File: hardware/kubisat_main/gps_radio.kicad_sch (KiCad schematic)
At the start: 10 parts, among them J1 IPX, U2 NEO-6M-GPS, U5 XL1278-SMT

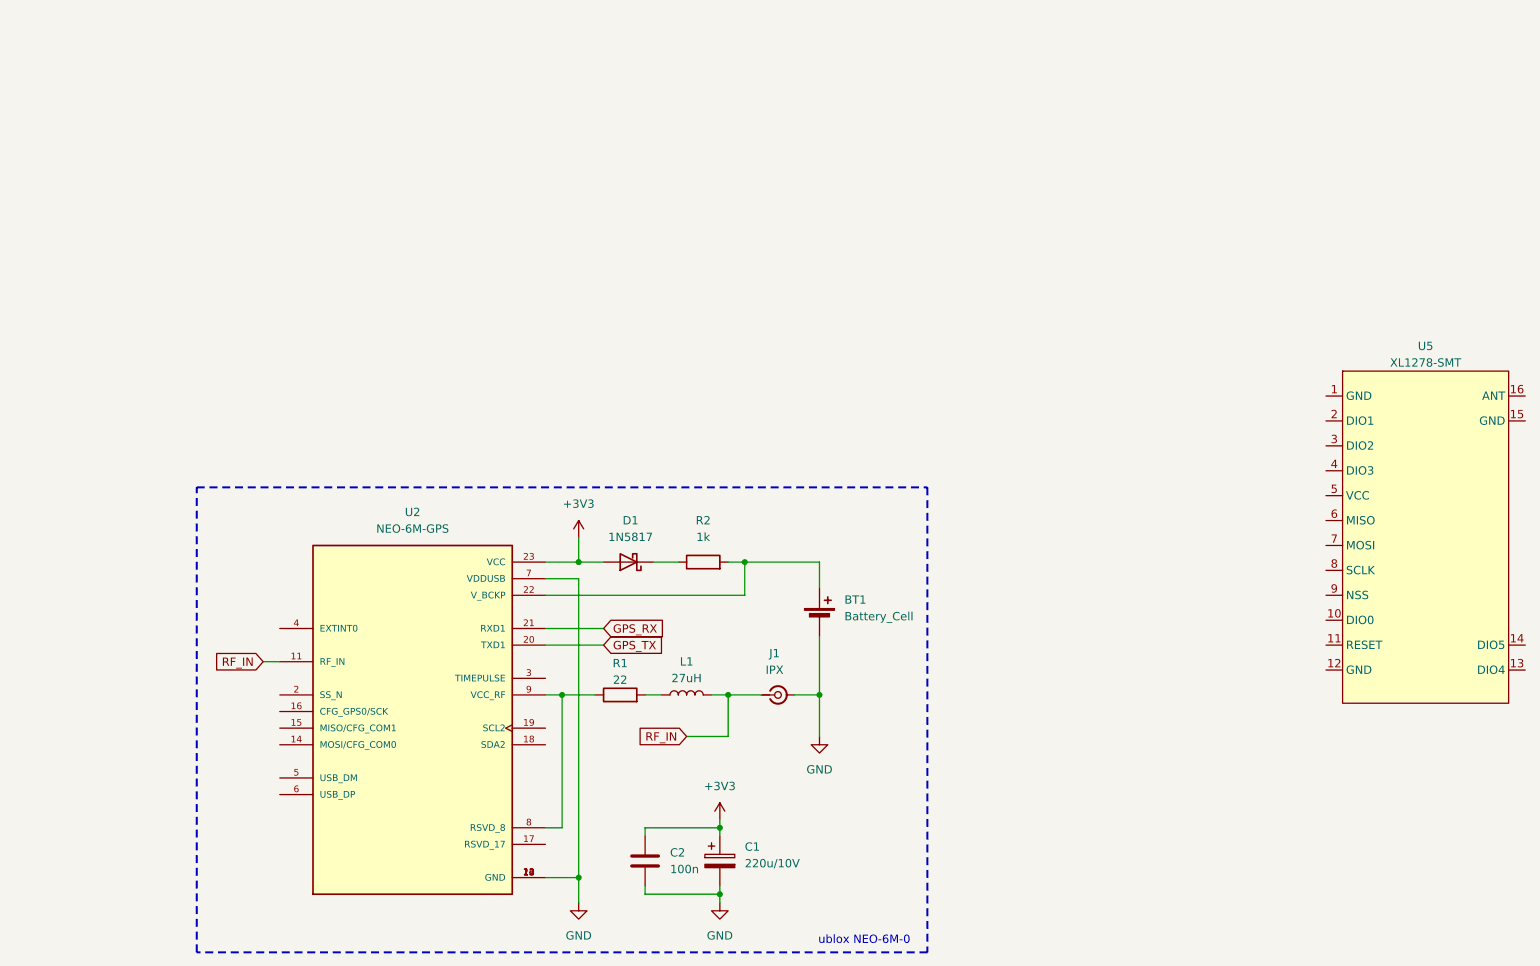
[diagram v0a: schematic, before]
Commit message: added elements to cpu schematic
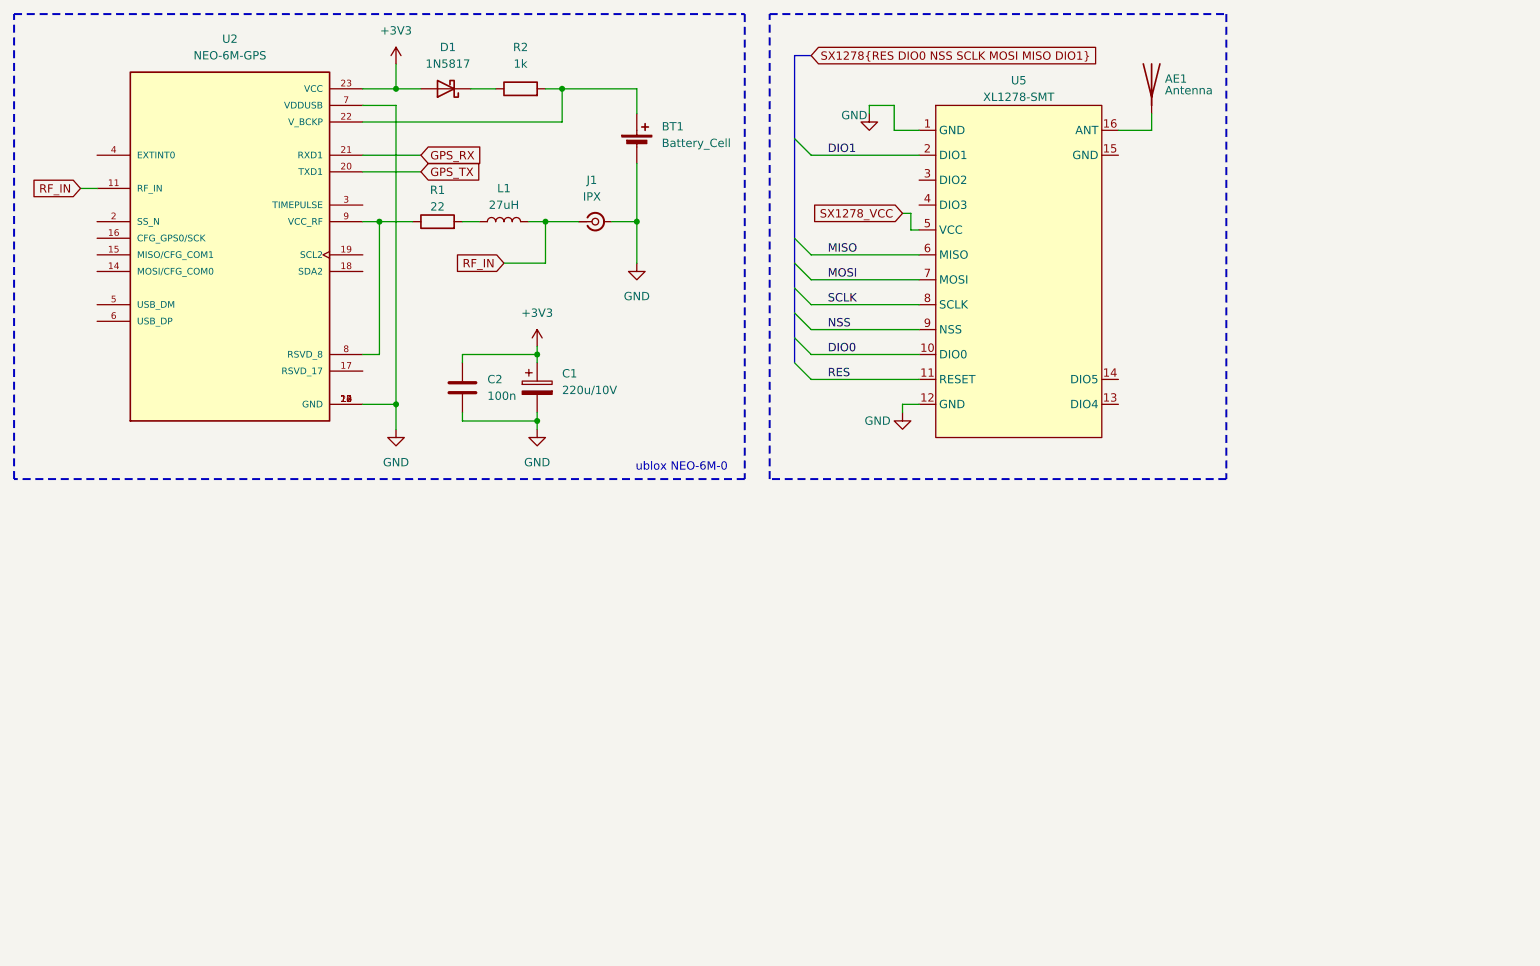
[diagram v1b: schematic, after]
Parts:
- added AE1: Antenna, symbol Device:Antenna
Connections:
- net GND: now also U5.1 (GND), U5.12 (GND)
- net DIO0: now reaches U5.10 (DIO0)
- net RES: now reaches U5.11 (RESET)
- net at U5.16 (ANT): now also AE1.1 (A)
- net DIO1: now reaches U5.2 (DIO1)
- net SX1278_VCC: now reaches U5.5 (VCC)
- net MISO: now reaches U5.6 (MISO)
- net MOSI: now reaches U5.7 (MOSI)
- net SCLK: now reaches U5.8 (SCLK)
- net NSS: now reaches U5.9 (NSS)
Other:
- moved on the sheet: BT1, C1, C2, D1, J1, L1, R1, R2, U2, U5

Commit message: changed strucutre, split main into 2 sseparate boards
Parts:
- removed AE1: Antenna, symbol Device:Antenna
- removed BT1: Battery_Cell, Battery:BatteryHolder_Seiko_MS621F, symbol Device:Battery_Cell
- removed C1: 220u/10V, Capacitor_Tantalum_SMD:CP_EIA-6032-15_Kemet-U, symbol Device:C_Polarized
- removed C2: 100n, Capacitor_SMD:C_0805_2012Metric, symbol Device:C
- removed D1: 1N5817, Diode_SMD:D_SOD-123, symbol Device:D_Schottky
- removed J1: IPX, Connector_Coaxial:U.FL_Hirose_U.FL-R-SMT-1_Vertical, symbol Connector:Conn_Coaxial_Small
- removed L1: 27uH, Inductor_SMD:L_0805_2012Metric, symbol Device:L
- removed R1: 22, Resistor_SMD:R_0805_2012Metric, symbol Device:R
- removed R2: 1k, Resistor_SMD:R_0805_2012Metric, symbol Device:R
- removed U2: NEO-6M-GPS, NEO-6M-GPS:XCVR_NEO-6M-GPS, symbol RF_GPS:NEO-6M-GPS
- removed U5: XL1278-SMT, RF:XL1278-SMT, symbol RF:XL1278-SMT
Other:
- note removed: "ublox NEO-6M-0"
